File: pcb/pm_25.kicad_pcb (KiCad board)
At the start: 2 copper layers, 50 x 38 mm, 19 parts, among them J1 USB_C_Receptacle_USB2.0, J2 header, J3 Qwiic, J4 Qwiic, U1 MCP1700, U2 MCP2221AxP, U3 ESP-12F, U4 PM2.5

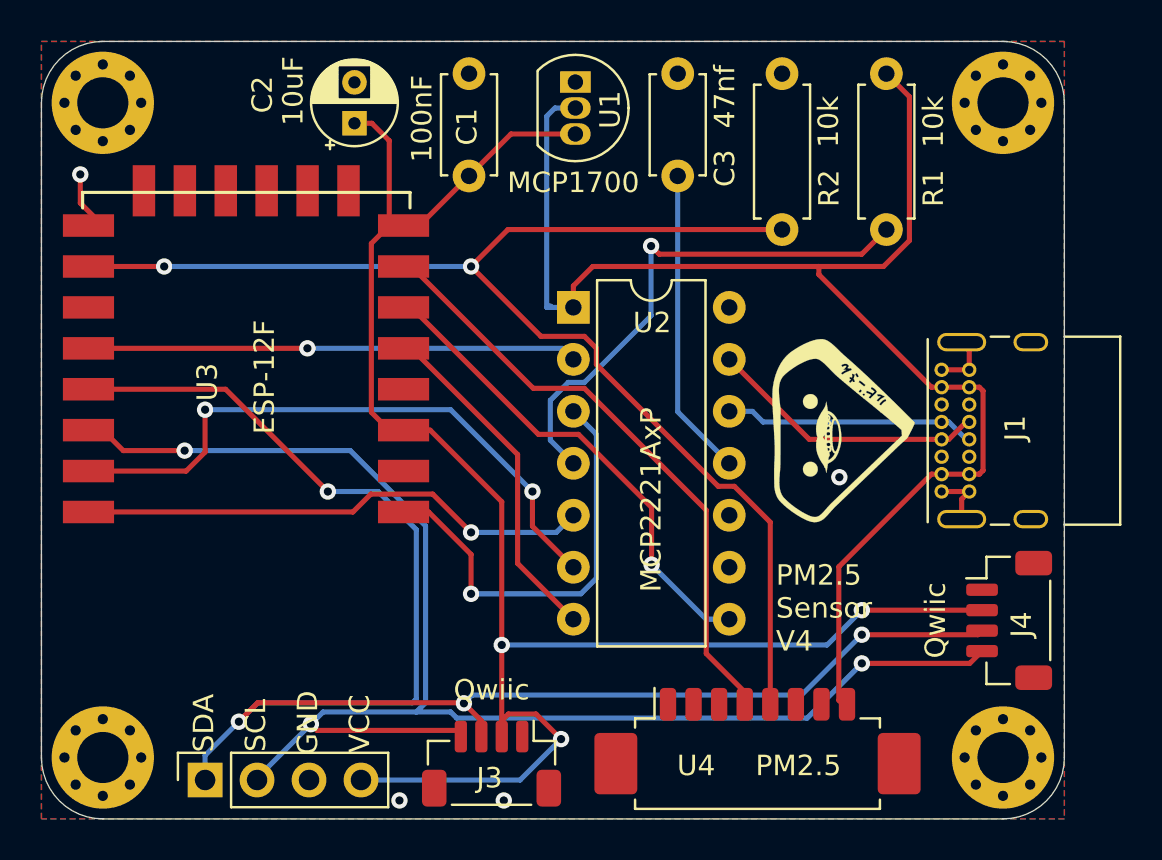
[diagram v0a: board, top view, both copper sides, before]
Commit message: updating PCB
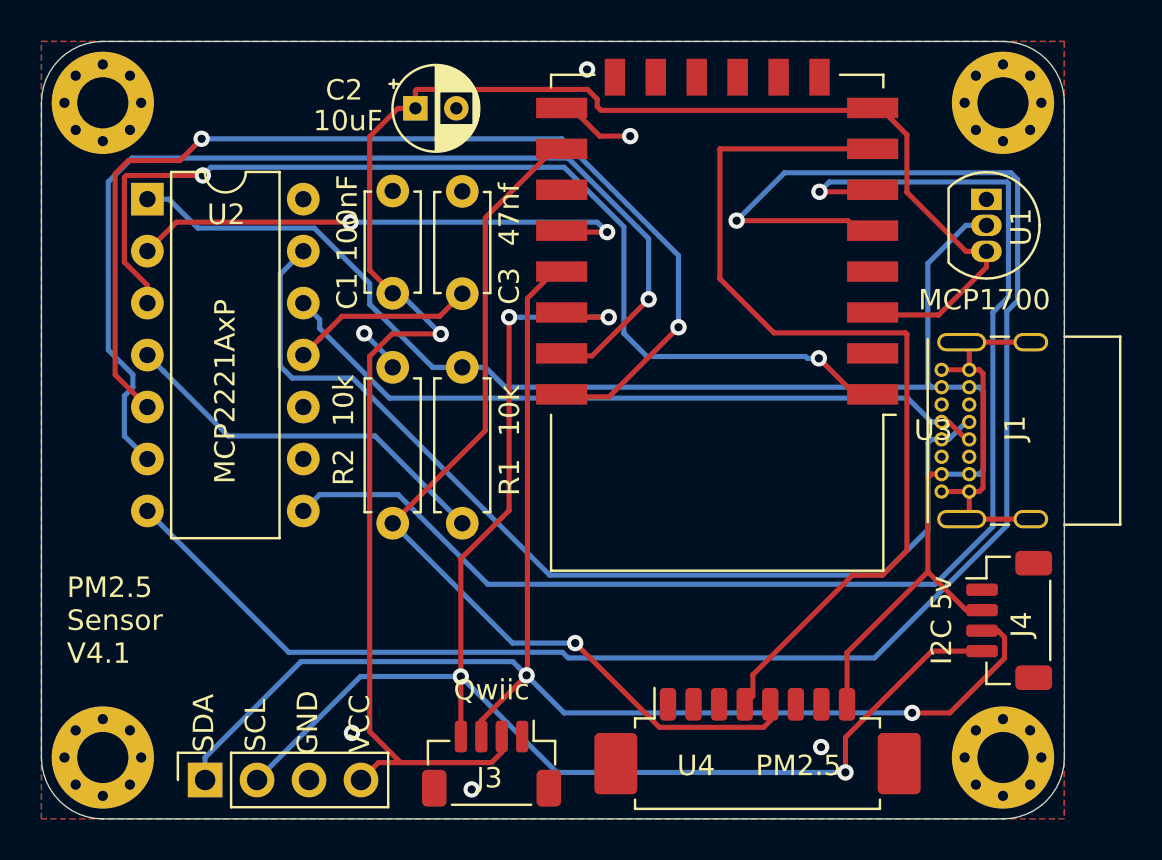
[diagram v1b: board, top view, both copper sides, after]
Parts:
- removed G***: LOGO, artwork:gorby
- removed G***: LOGO, artwork:rubysan
- J4: value Qwiic -> I2C 5v
- U3: footprint ESP8266:ESP-12E_SMD -> RF_Module:ESP-12E
- moved R1 25.2 mm to (130.6, 85.9)
- moved R2 23.8 mm to (127.2, 93.5)
- moved U2 21.5 mm to (115.2, 77.7)
- moved U1 20.9 mm to (156.2, 77.7)
- moved U3 18.5 mm to (143.0, 83.8)
- moved C3 12.0 mm to (130.6, 77.3)
- moved C1 6.84 mm to (127.2, 82.3)
- moved C2 3.07 mm to (128.3, 73.3), turned to 0 degrees
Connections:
- J4 pad 2: +3V3 -> +5V
- U3 pad 10: Net-(R2-Pad1) -> (no net)
- U3 pad 12: /FLASH -> (no net)
- U3 pad 13: /SDA -> (no net)
- U3 pad 14: /SCL -> (no net)
- U3 pad 15: Net-(U2-Pad6) -> GND
- U3 pad 16: Net-(U2-Pad5) -> Net-(R2-Pad1)
- U3 pad 18: (no net) -> /FLASH
- U3 pad 19: (no net) -> /SDA
- U3 pad 20: (no net) -> /SCL
- U3 pad 21: (no net) -> Net-(U2-Pad6)
- U3 pad 22: (no net) -> Net-(U2-Pad5)
- U3 pad 9: GND -> (no net)
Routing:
- net Net-(U2-Pad7): track 17.6 -> 85.9 mm, vias 0 -> 1
- net Net-(U2-Pad8): track 24.6 -> 65.6 mm
- net /D+: track 13.7 -> 49.6 mm
- net /RST: track 21.9 -> 50.5 mm, vias 1 -> 2
- net Net-(U2-Pad5): track 24.5 -> 52.7 mm, vias 1 -> 2
- net /D-: track 12.3 -> 35.6 mm
- net Net-(U2-Pad6): track 29.6 -> 51.0 mm, vias 2 -> 1
- net Net-(R2-Pad1): track 63.4 -> 46.0 mm, vias 2 -> 1
- net GND: track 8.66 -> 25.1 mm, vias 4 -> 6
- net Net-(U3-Pad7): track 30.9 -> 45.8 mm
- net +5V: track 70.1 -> 78.0 mm
- net /SDA: track 79.2 -> 71.6 mm, vias 4 -> 2
- net Net-(R1-Pad2): track 25.8 -> 18.8 mm, vias 1 -> 0
- net Net-(C3-Pad2): track 15.1 -> 9.01 mm
- net +3V3: track 85.1 -> 88.6 mm, vias 3 -> 1
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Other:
- board text added: "PM2.5 Sensor V4.1"
- board text removed: "PM2.5 Sensor V4"
